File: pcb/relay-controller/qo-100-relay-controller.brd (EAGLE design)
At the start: 85 x 83.8 mm, 134 parts, among them CON1 4P-SH-SIDE, CON10 2EDG-2P-5MM, CON11 2EDG-2P-5MM, CON12 2EDG-2P-5MM, CON13 2EDG-2P-5MM, CON14 2EDG-2P-5MM, CON2 2EDG-2P-5MM, CON3 2EDG-2P-5MM, CON4 2EDG-2P-5MM, CON5 2EDG-2P-5MM, CON6 2EDG-2P-5MM, CON7 2EDG-2P-5MM, CON8 2EDG-2P-5MM, CON9 2EDG-2P-5MM, Q1 AO3400, Q10 AO3400, Q11 AO3400, Q12 AO3400, Q2 AO3400, Q3 AO3400, Q4 AO3400, Q5 AO3400, Q6 AO3400, Q7 AO3400, Q8 AO3400, Q9 AO3400, U1 MCP1792-3.3, U2 EFM32TG11B120F128GM32

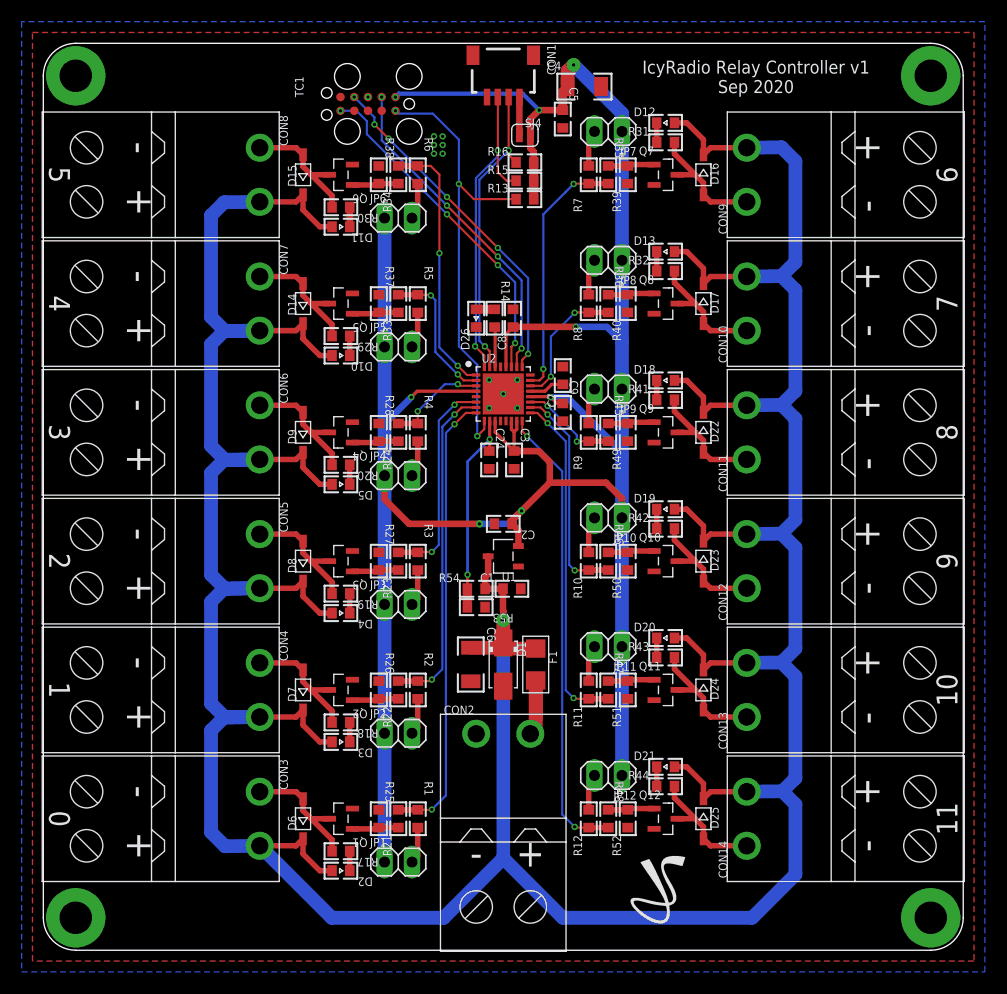
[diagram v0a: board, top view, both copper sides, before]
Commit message: Work on PCBs
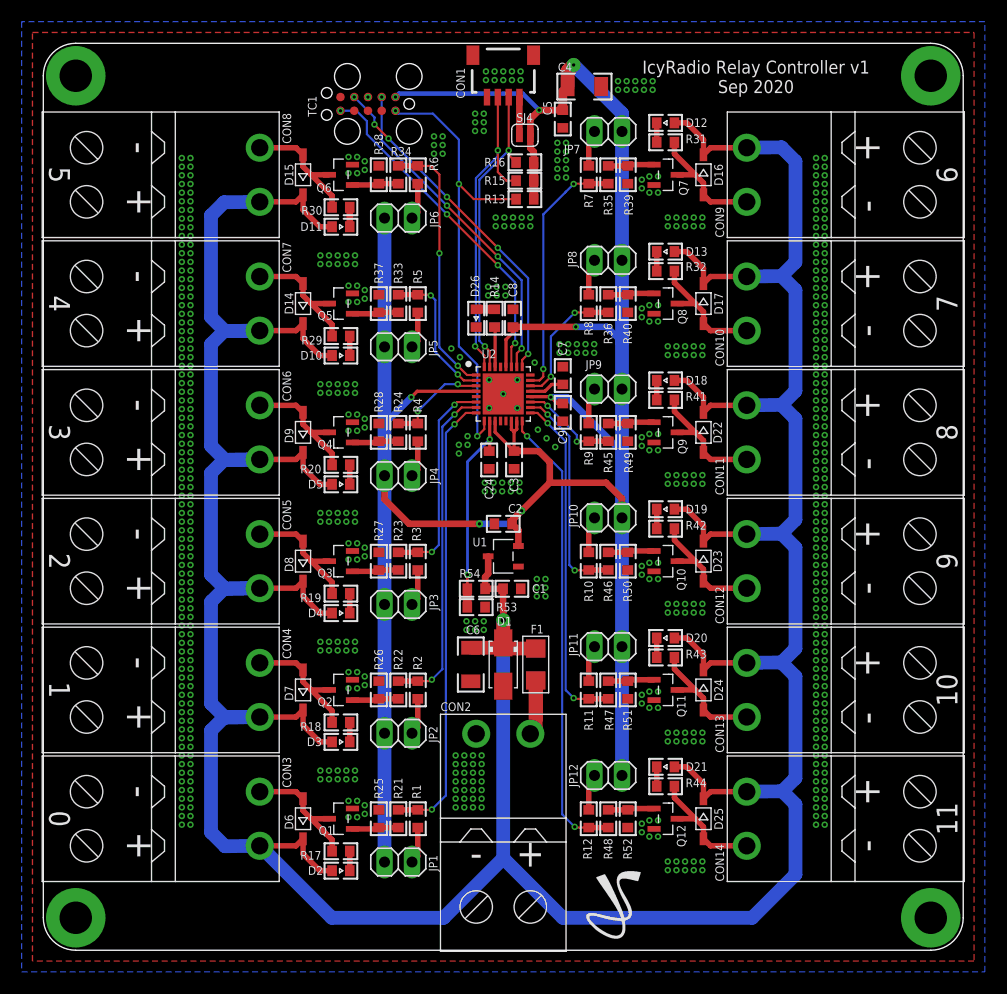
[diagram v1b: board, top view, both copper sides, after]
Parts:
- moved LOGO1 4.33 mm to (55.4, 7.50)
